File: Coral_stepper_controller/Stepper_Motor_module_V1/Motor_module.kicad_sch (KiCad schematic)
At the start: 34 parts, among them J1 Limit Switch, J2 Limit Switch, J3 Limit Switch, J4 Limit Switch, J5 Conn_01x08_Male, J6 Conn_01x04_Male, J7 Conn_01x08_Female, J8 Conn_01x08_Female, SW1 SW_Push, U1 STM32F031F6P6, Y1 8MHz

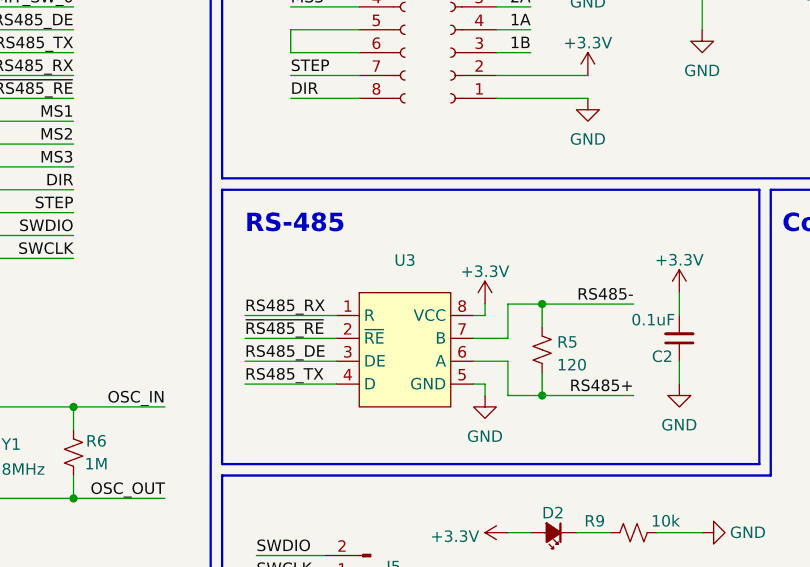
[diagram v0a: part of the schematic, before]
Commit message: udated by FZ
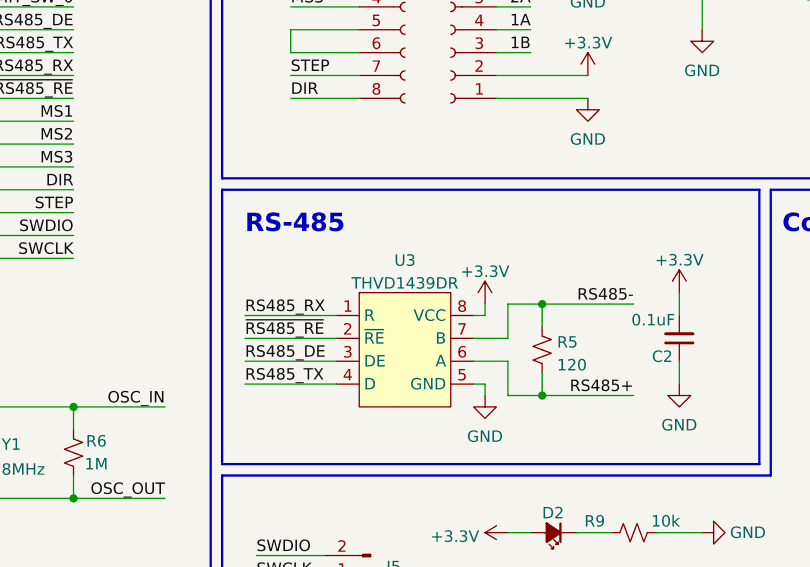
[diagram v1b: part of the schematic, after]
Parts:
- U3: value (none) -> THVD1439DR
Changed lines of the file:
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@@
     (in_bom yes) (on_board yes) (fields_autoplaced)
     (property "Reference" "U3" (id 0) (at 110.49 63.7372 0))
-    (property "Value" "" (id 1) (at 110.49 66.2741 0))
+    (property "Value" "THVD1439DR" (id 1) (at 110.49 66.2741 0))
     (property "Footprint" "Package_SO:PowerIntegrations_SO-8" (id 2) (at 110.49 63.5 0)
       (effects (font (size 1.27 1.27)) hide)

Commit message: udated by FZ
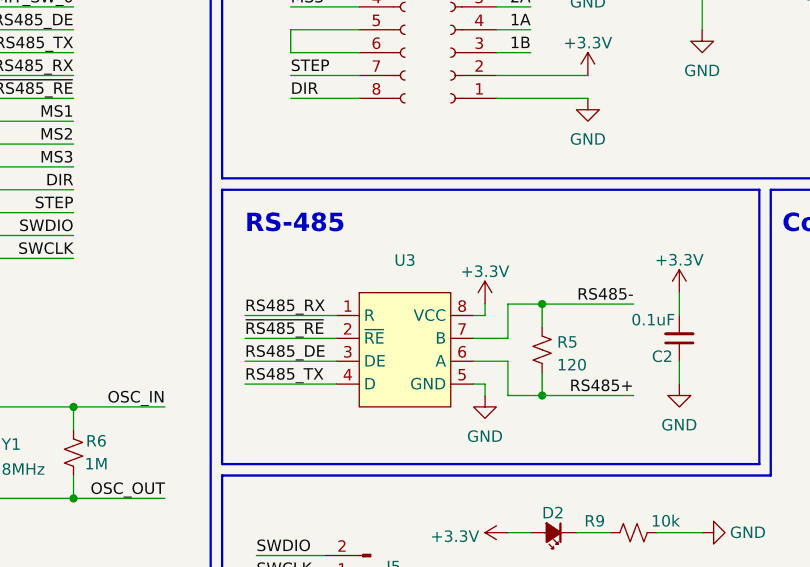
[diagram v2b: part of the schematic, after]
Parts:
- U3: value THVD1439DR -> (none)
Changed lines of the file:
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@@
     (in_bom yes) (on_board yes) (fields_autoplaced)
     (property "Reference" "U3" (id 0) (at 110.49 63.7372 0))
-    (property "Value" "THVD1439DR" (id 1) (at 110.49 66.2741 0))
+    (property "Value" "" (id 1) (at 110.49 66.2741 0))
     (property "Footprint" "Package_SO:PowerIntegrations_SO-8" (id 2) (at 110.49 63.5 0)
       (effects (font (size 1.27 1.27)) hide)
